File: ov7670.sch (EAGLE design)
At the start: 3 parts

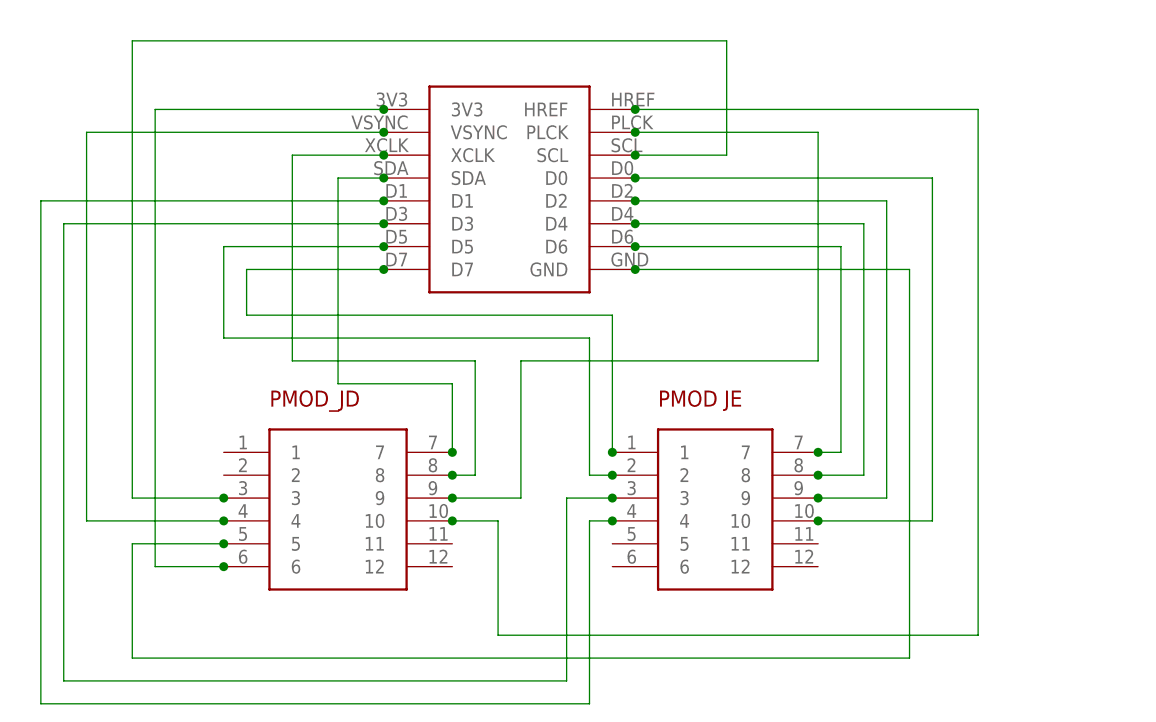
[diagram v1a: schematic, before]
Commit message: temporal commit
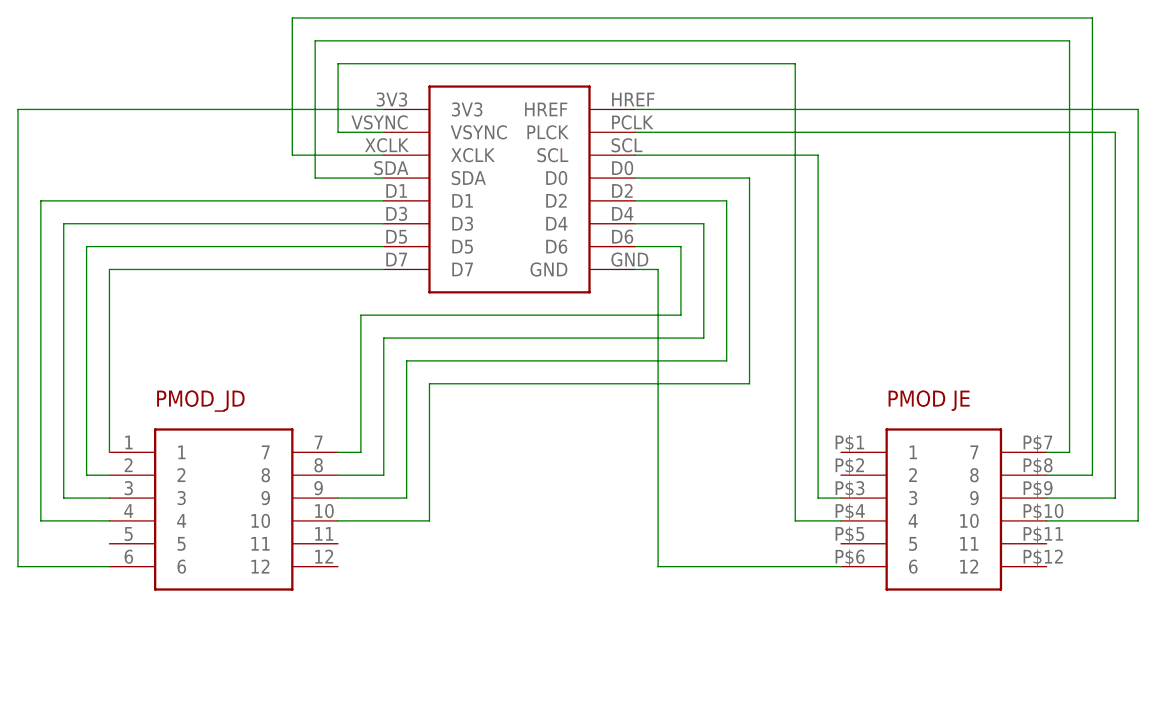
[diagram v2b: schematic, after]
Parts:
- renumbered U$1 to D6
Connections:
- removed net D6: D6.D6, U$3.7
- removed net GND: D6.GND, U$2.5
- removed net PLCK: D6.PLCK, U$2.9
- new net N$1: D6.GND, U$3.6
- new net N$6: D6.D6, U$2.7
- new net PCLK: D6.PLCK, U$3.9
- net D0: now also U$2.10; no longer U$3.10
- net D1: now also U$2.4; no longer U$3.4
- net D2: now also U$2.9; no longer U$3.9
- net D3: now also U$2.3; no longer U$3.3
- net D4: now also U$2.8; no longer U$3.8
- net D5: now also U$2.2; no longer U$3.2
- net D7: now also U$2.1; no longer U$3.1
- net HREF: now also U$3.10; no longer U$2.10
- net SCL: now also U$3.3; no longer U$2.3
- net SDA: now also U$3.7; no longer U$2.7
- net VSYNC: now also U$3.4; no longer U$2.4
- net XCLK: now also U$3.8; no longer U$2.8

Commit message: update
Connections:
- net N$1 renamed GND
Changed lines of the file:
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@@
 </segment>
 </net>
-<net name="N$1" class="0">
+<net name="GND" class="0">
 <segment>
 <pinref part="D6" gate="G$1" pin="GND"/>
